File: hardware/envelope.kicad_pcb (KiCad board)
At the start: 4 copper layers, 86 x 99 mm, 57 parts, among them J1 Barrel_Jack_Switch_MountingPin, J2 AudioJack3_Switch, J3 AudioJack3_Switch, SW1 SW_DPDT_x2, SW2 SW_SPDT, U1 4066, U2 4069, U3 4069

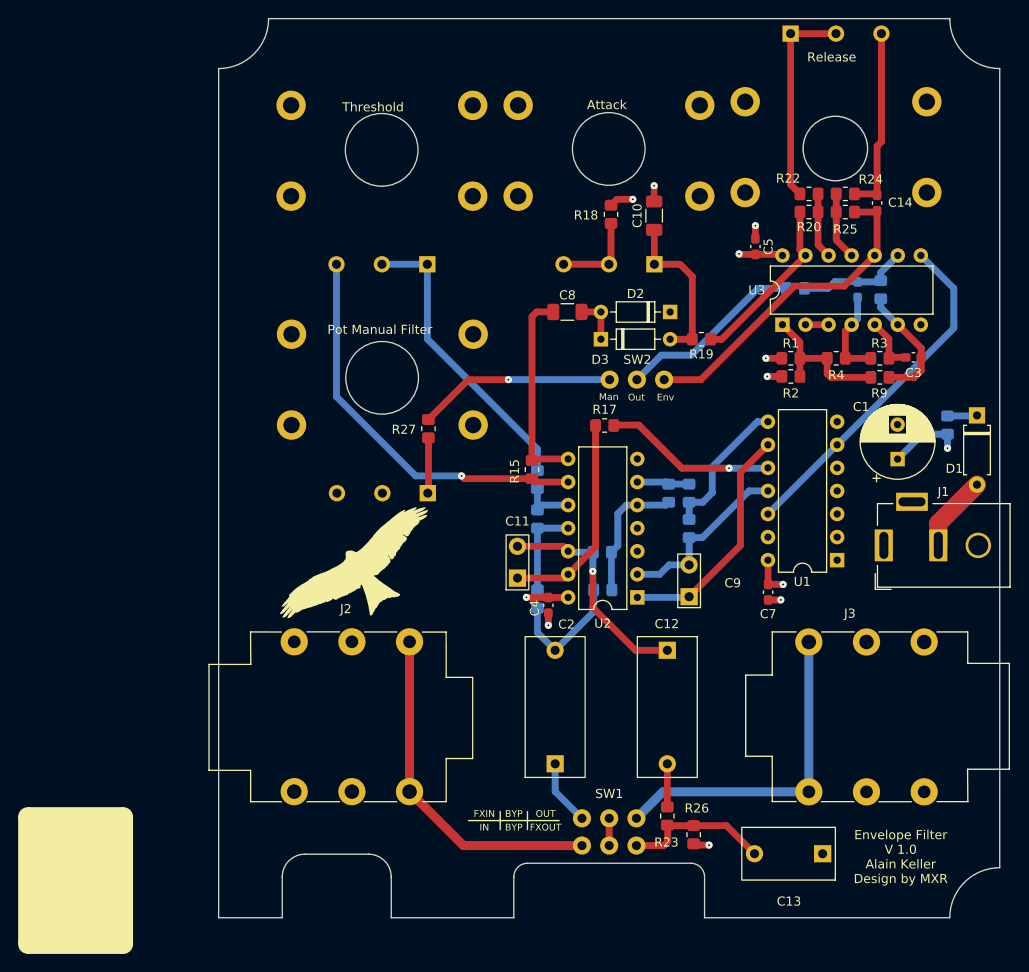
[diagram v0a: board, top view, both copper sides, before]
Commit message: pre via stitch
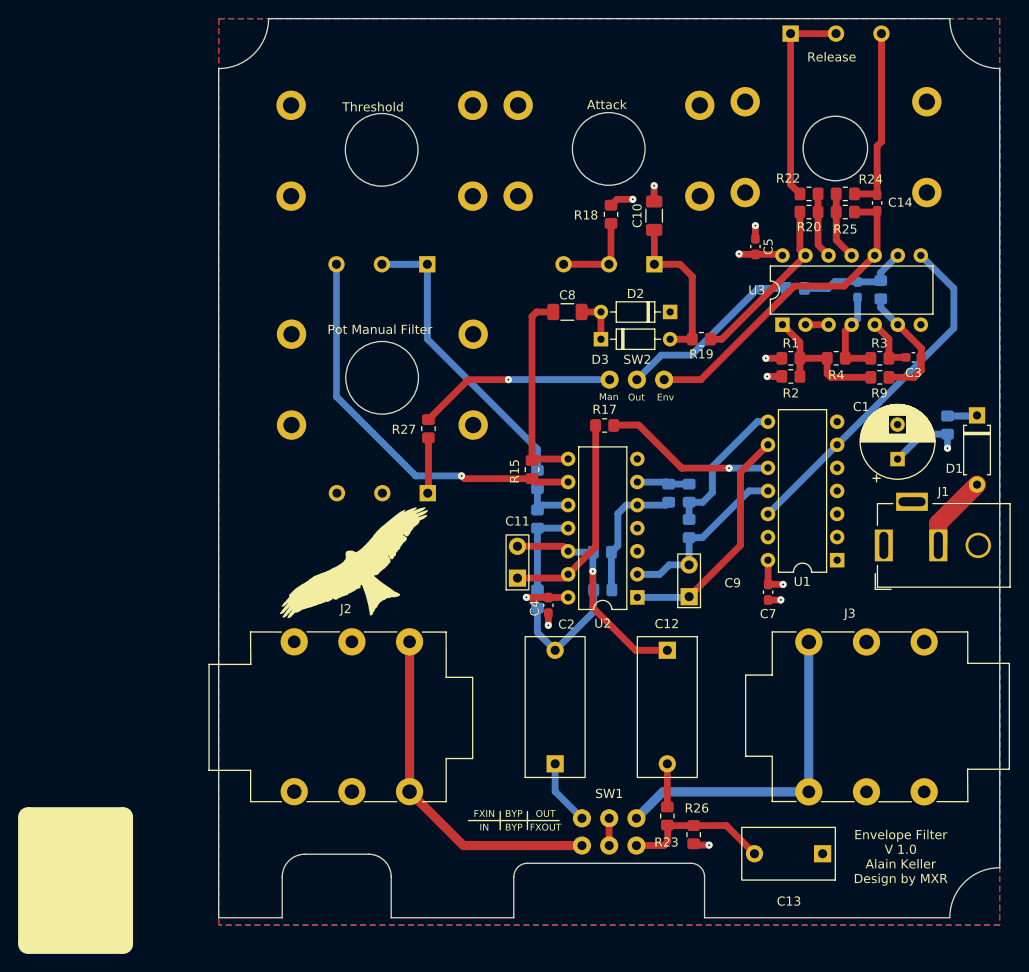
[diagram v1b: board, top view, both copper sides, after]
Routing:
- added copper zone on B.Cu, net GND
- added copper zone on F.Cu, net GND
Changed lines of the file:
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@@
     (56 "User.7" user)
     (57 "User.8" user)
-    (58 "User.9" user)
+    (58 "User.9" user "plugins.config")
   )
   (setup
@@
   (segment (start 179.2375 85.5725) (end 183.5 81.31) (width 2) (layer "F.Cu") (net 53))
   (segment (start 179.2375 88) (end 179.2375 85.5725) (width 2) (layer "F.Cu") (net 53))
-  (zone (net 1) (net_name "VS") (layer "In1.Cu") (hatch edge 0.508)
+  (zone (net 2) (net_name "GND") (layers F&B.Cu) (hatch edge 0.508)
     (connect_pads (clearance 0))
     (min_thickness 0.254) (filled_areas_thickness no)
-    (fill yes (thermal_gap 0.508) (thermal_bridge_width 0.508))
+    (fill yes (mode hatch) (thermal_gap 0.508) (thermal_bridge_width 0.508)
+      (hatch_thickness 0.716) (hatch_gap 1.524) (hatch_orientation 45)
+      (hatch_border_algorithm hatch_thickness) (hatch_min_hole_area 0.3))
     (polygon
       (pts
         (xy 186 30)
         (xy 186 80)
-        (xy 186 134.5)
-        (xy 100 134.5)
+        (xy 186 129.8)
+        (xy 100 129.8)
         (xy 100 55)
         (xy 100 30)
@@
     )
   )
-  (zone (net 2) (net_name "GND") (layer "In2.Cu") (hatch edge 0.508)
+  (zone (net 1) (net_name "VS") (layer "In1.Cu") (hatch edge 0.508)
     (connect_pads (clearance 0))
     (min_thickness 0.254) (filled_areas_thickness no)
